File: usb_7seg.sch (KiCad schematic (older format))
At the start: 8 parts, among them IC1 MAX7219CNG, IC2 MAX7219CWG, U1 SeeeduinoXIAO, U2 7segment_led

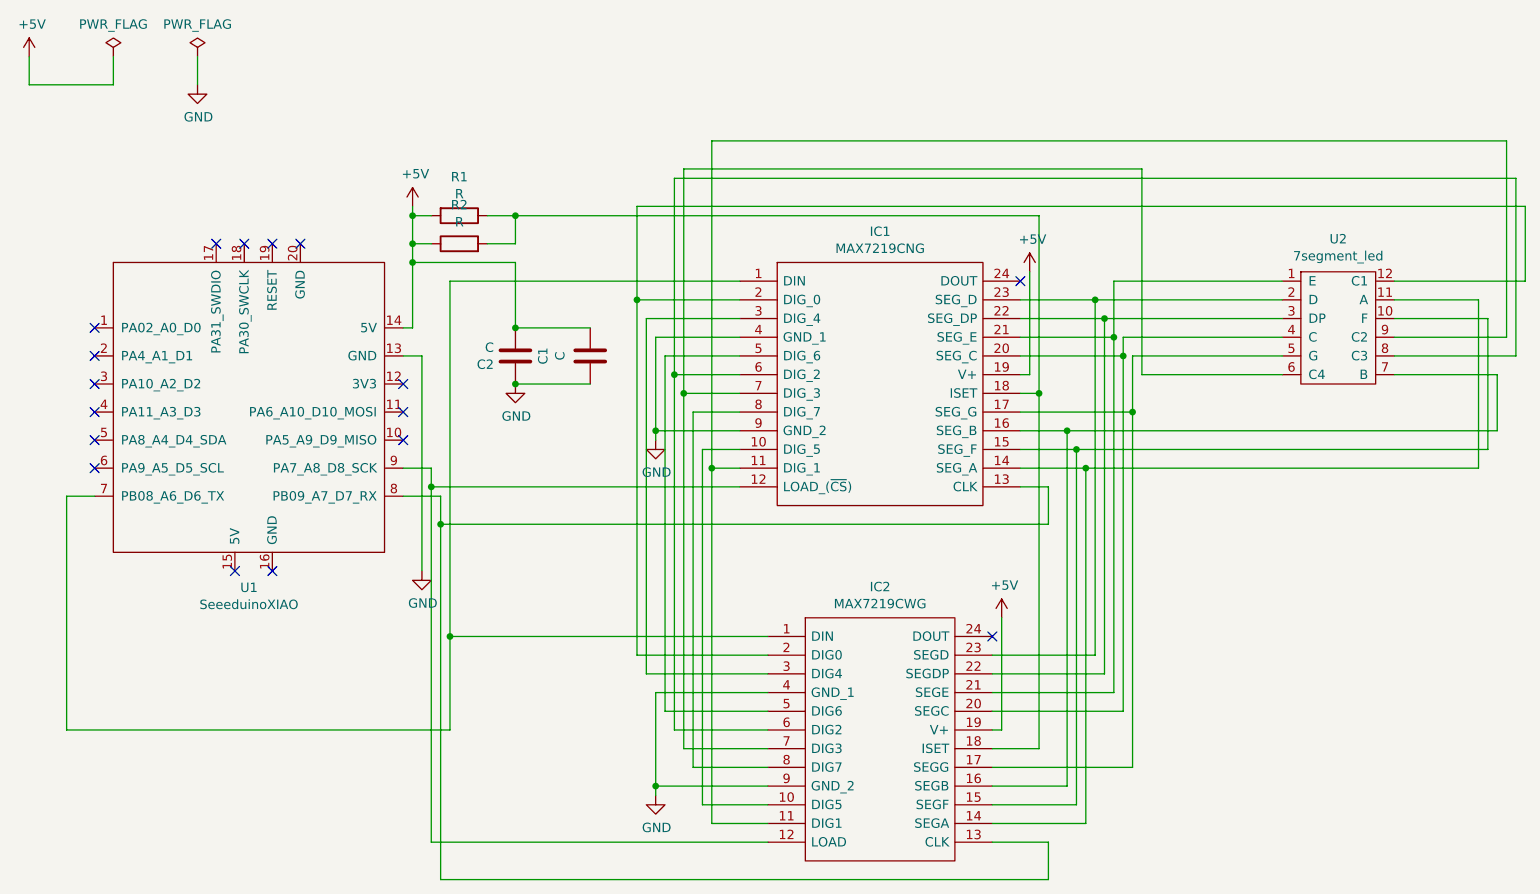
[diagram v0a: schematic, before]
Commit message: 配置配線、ERC ok
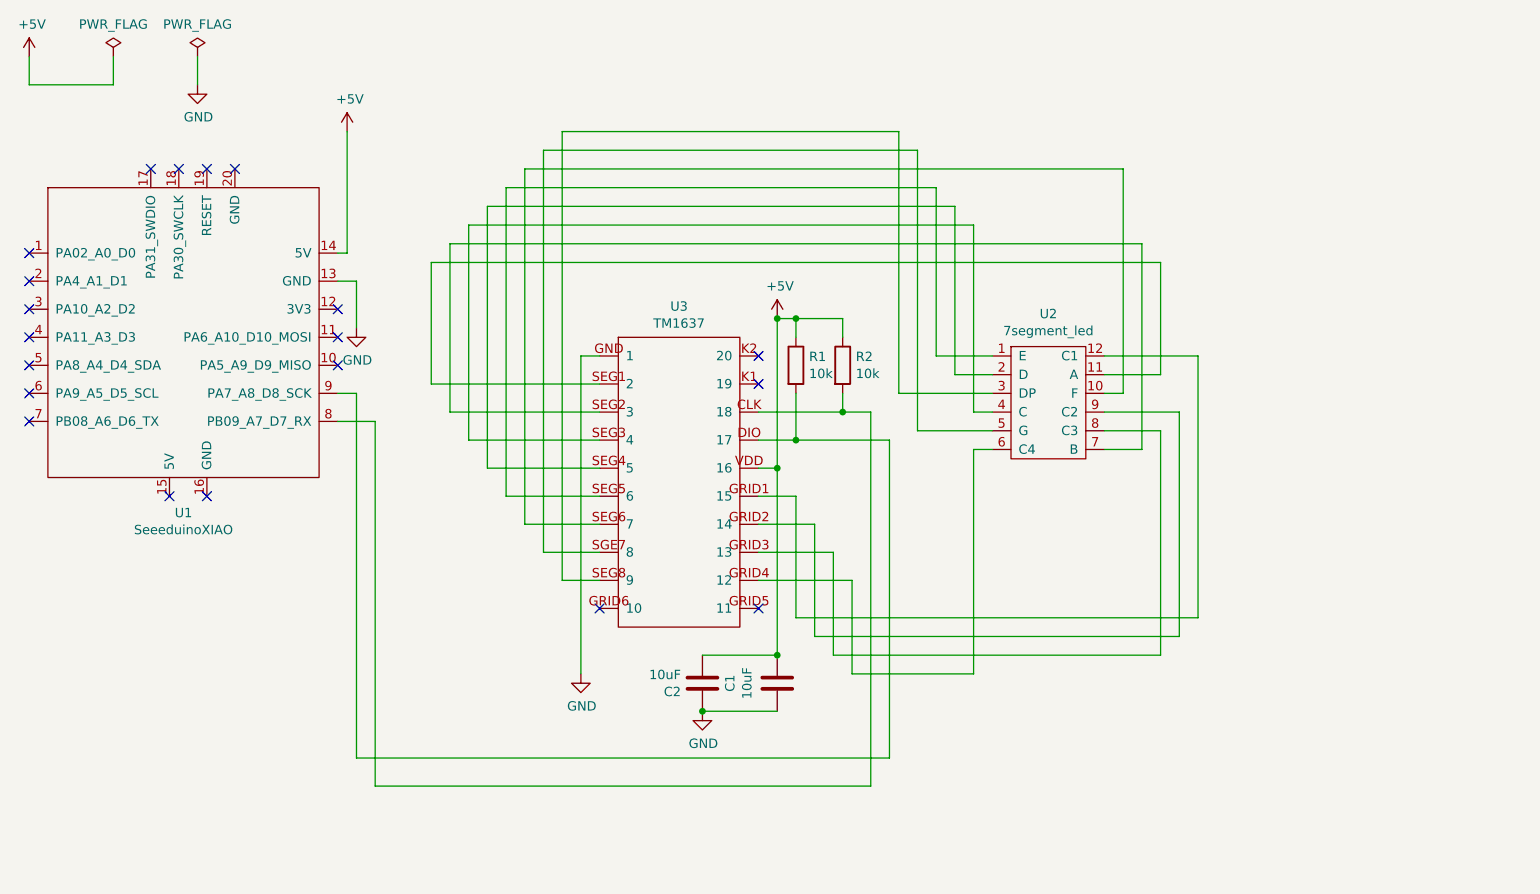
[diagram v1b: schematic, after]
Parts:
- removed IC1: MAX7219CNG, MAX7219CNG:MAX7219CNG, symbol MAX7219CNG:MAX7219CNG
- removed IC2: MAX7219CWG, MAX7219CWG:MAX7219CWG, symbol MAX7219CWG:MAX7219CWG
- added U3: TM1637, kicad_mylib:TM1630, symbol kicad_mylib:TM1637
- C1, C2: value C -> 10uF
- R1: value R -> 10k
- R2: value R -> 10k; footprint Resistor_SMD:R_0805_2012Metric_Pad1.15x1.40mm_HandSolder -> Resistor_THT:R_Axial_DIN0207_L6.3mm_D2.5mm_P10.16mm_Horizontal
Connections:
- net +5V: now also R1.1, U3.VDD (16); no longer R1.2
- net GND: now also U3.GND (1)
- net at U2.9 (C2): now also U3.GRID2 (14)
- net at U1.9 (PA7_A8_D8_SCK): now also R1.2, U3.DIO (17)
- net at U1.8 (PB09_A7_D7_RX): now also R2.2, U3.CLK (18)
- net at U2.11 (A): now also U3.SEG1 (2)
- net at U2.10 (F): now also U3.SEG6 (7)
- net at U2.7 (B): now also U3.SEG2 (3)
- net at U2.5 (G): now also U3.SGE7 (8)
- net at U2.12 (C1): now also U3.GRID1 (15)
- net at U2.4 (C): now also U3.SEG3 (4)
- net at U2.1 (E): now also U3.SEG5 (6)
- net at U2.3 (DP): now also U3.SEG8 (9)
- net at U2.2 (D): now also U3.SEG4 (5)
- net at U2.8 (C3): now also U3.GRID3 (13)
- net at U2.6 (C4): now also U3.GRID4 (12)
- no-connect marks 17 -> 20
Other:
- moved on the sheet: C1, C2, U1, U2
